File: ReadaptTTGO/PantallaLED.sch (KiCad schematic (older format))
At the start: 20 parts, among them U7 662k, U8 OLED-128O064D

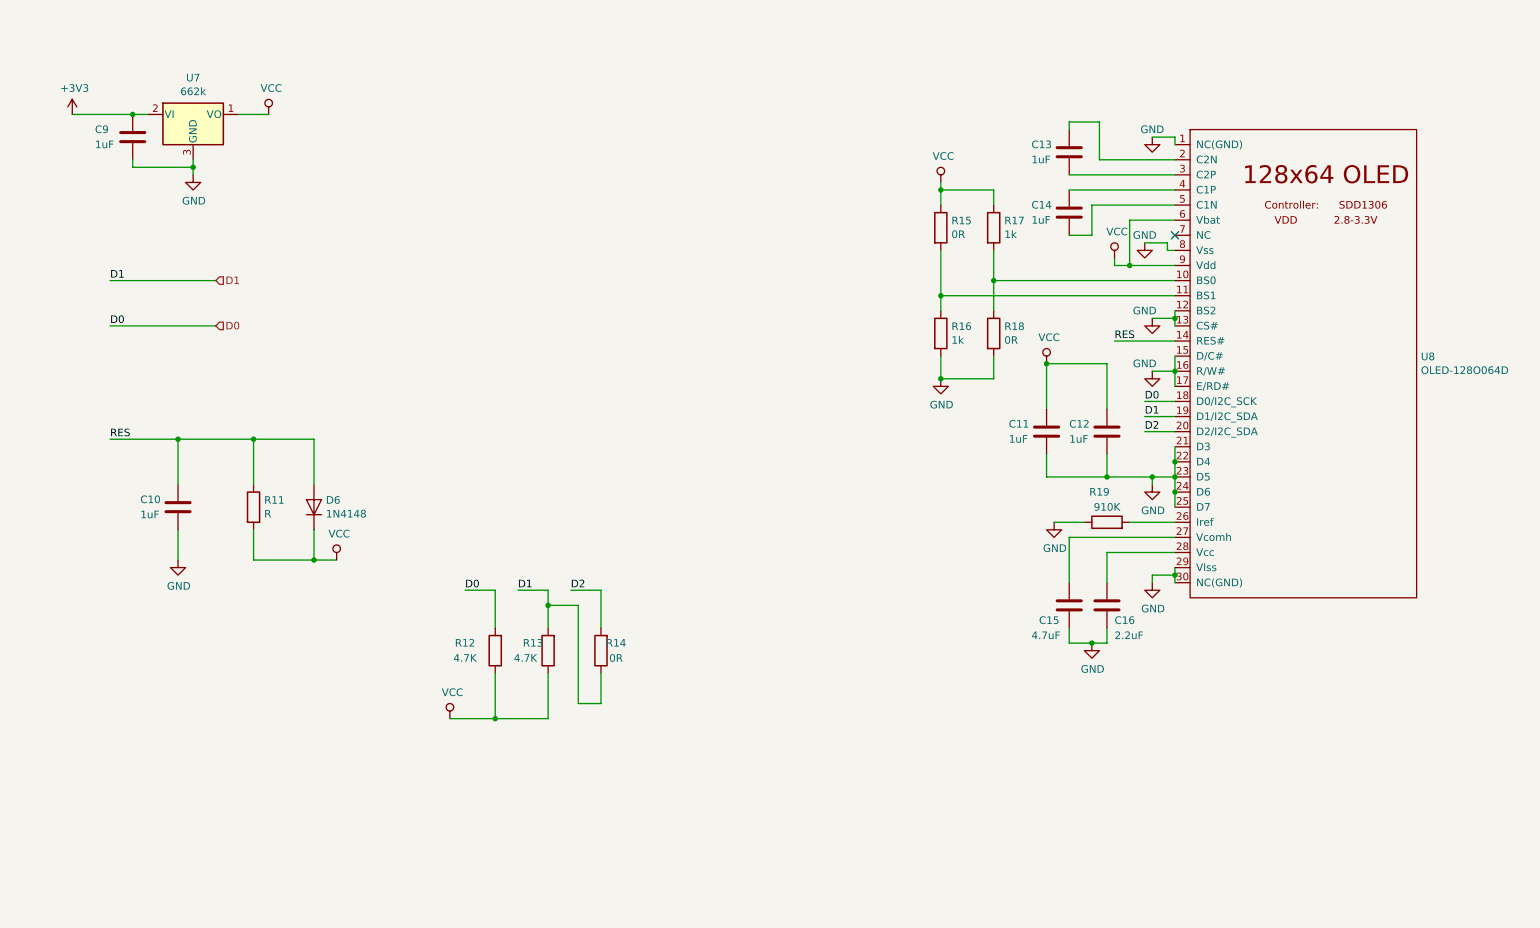
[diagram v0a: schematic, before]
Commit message: Entrega revision 1.2
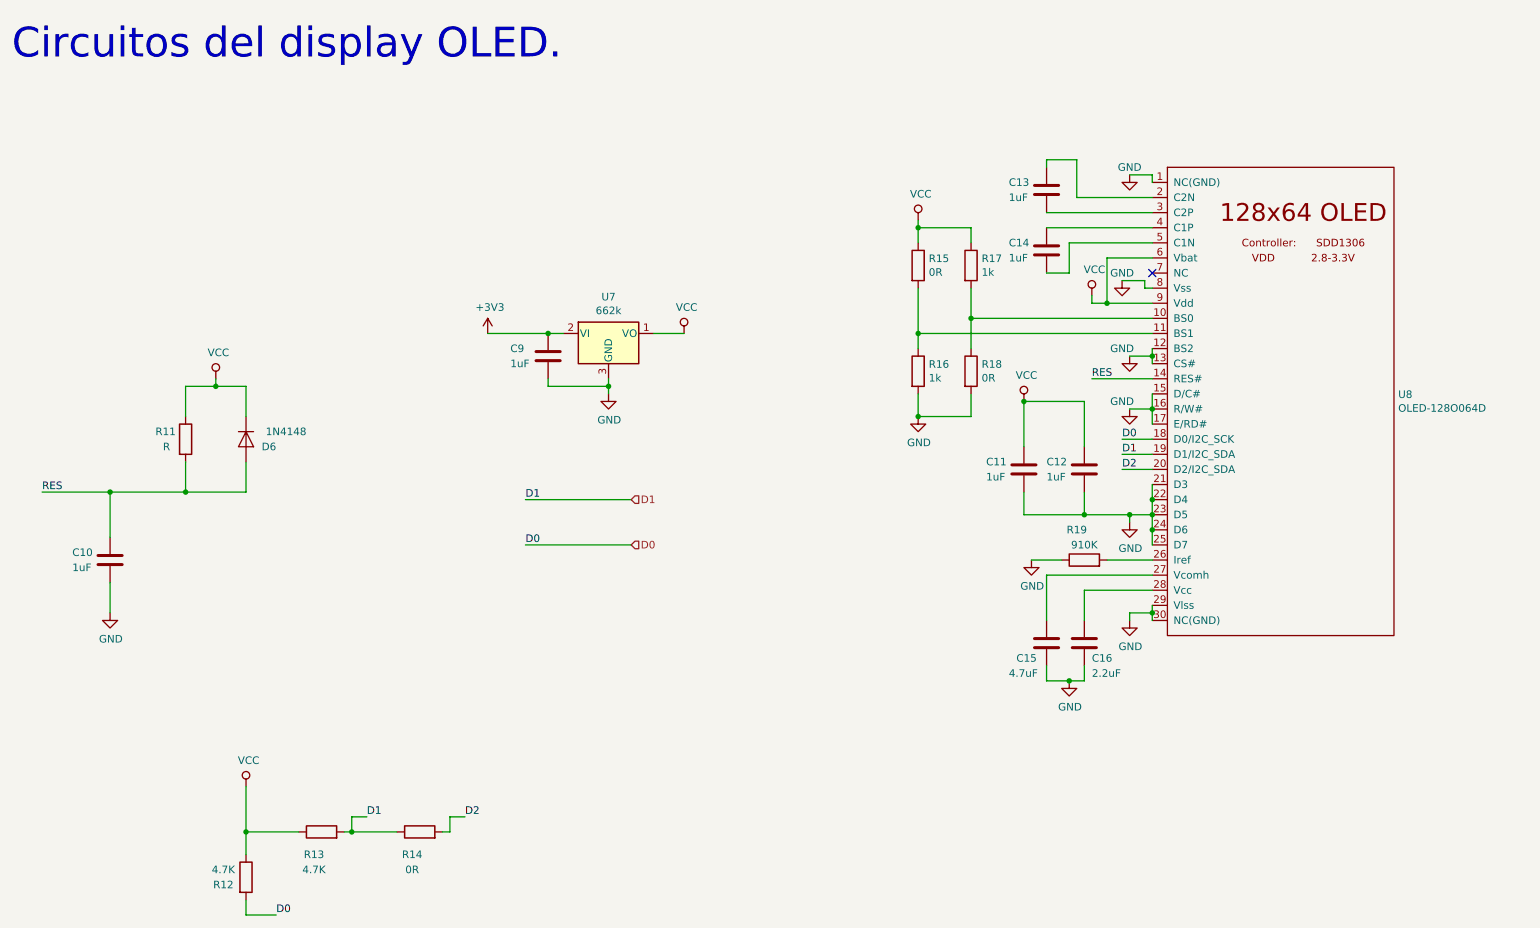
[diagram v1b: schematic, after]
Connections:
- net RES: now also R11.2; no longer R11.1
- net VCC: now also R11.1; no longer R11.2
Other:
- note added: "Circuitos del display OLED."
- moved on the sheet: C11, C12, C13, C14, C15, C16, C9, R15, R16, R17, R18, R19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
